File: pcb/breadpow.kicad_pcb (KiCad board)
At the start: 2 copper layers, 53.3 x 21.6 mm, 15 parts, among them J1 HRO 31-M-12, J2 Conn_01x02_Pin, J3 Conn_01x02_Pin, SW1 SW_DIP_x03, U1 CH224K

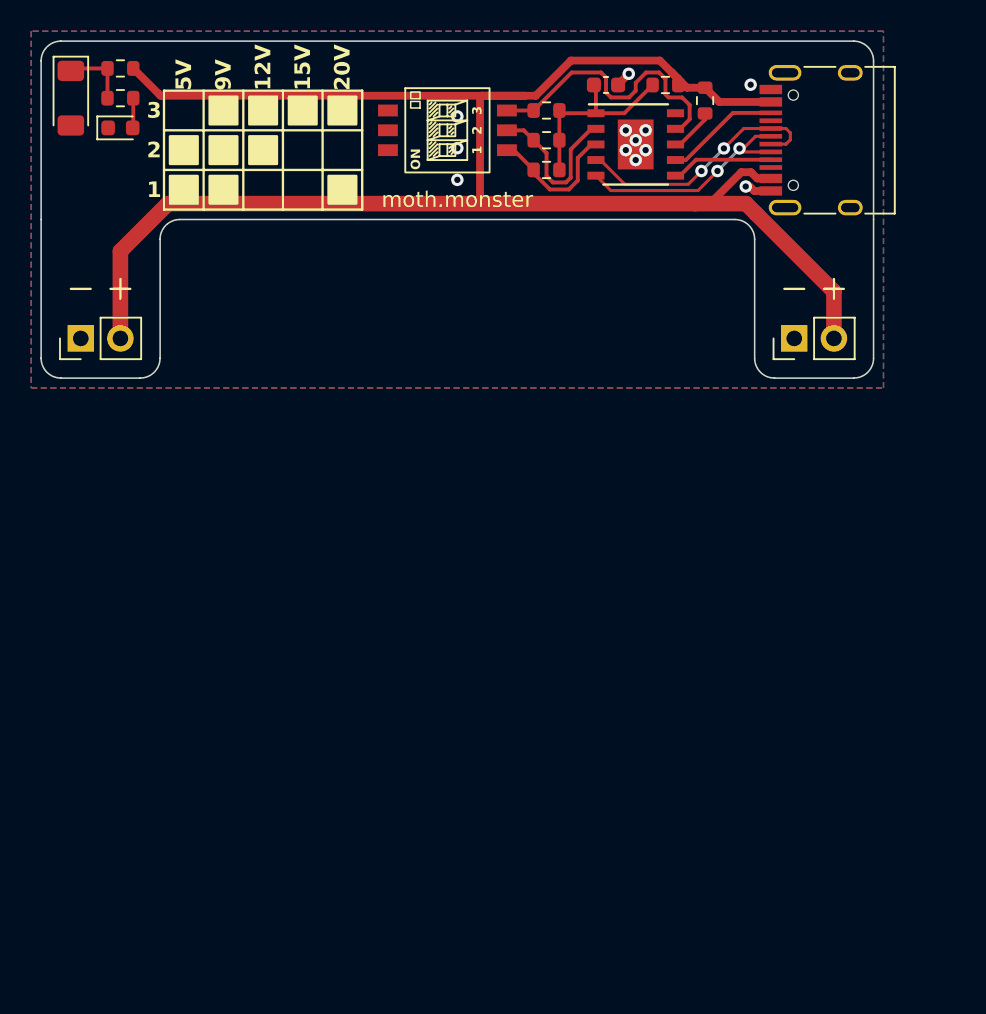
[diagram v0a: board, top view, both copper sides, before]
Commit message: forgot to add that
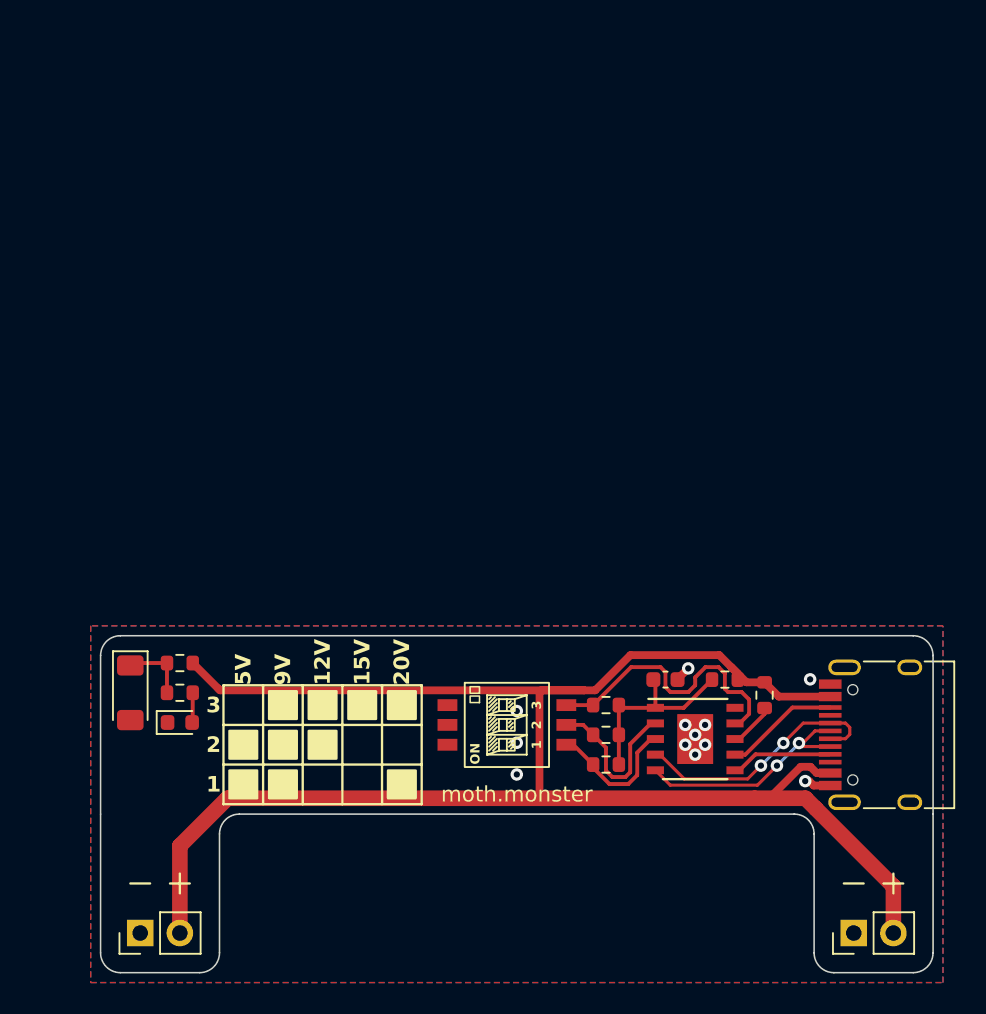
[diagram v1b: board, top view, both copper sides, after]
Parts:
- moved SW1 38.3 mm to (151.8, 95.9)
- moved U1 38.3 mm to (163.8, 96.8)
- moved C1 38.3 mm to (161.9, 93.0)
- moved D1 38.3 mm to (130.8, 95.7)
- moved D2 38.3 mm to (127.6, 93.8)
- moved R1 38.3 mm to (165.7, 93.0)
- moved R2 38.3 mm to (168.3, 94.0)
- moved R6 38.3 mm to (130.8, 91.9)
- moved R7 38.3 mm to (130.8, 93.8)
- moved J1 38.3 mm to (176.5, 96.5)
- moved J2 38.3 mm to (128.3, 109.2)
- moved J3 38.3 mm to (174.0, 109.2)
- moved R3 38.3 mm to (158.1, 94.6)
- moved R4 38.3 mm to (158.1, 96.5)
- moved R5 38.3 mm to (158.1, 98.4)
